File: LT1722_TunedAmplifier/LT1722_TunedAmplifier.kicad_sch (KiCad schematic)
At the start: 18 parts, among them U2 LT1722

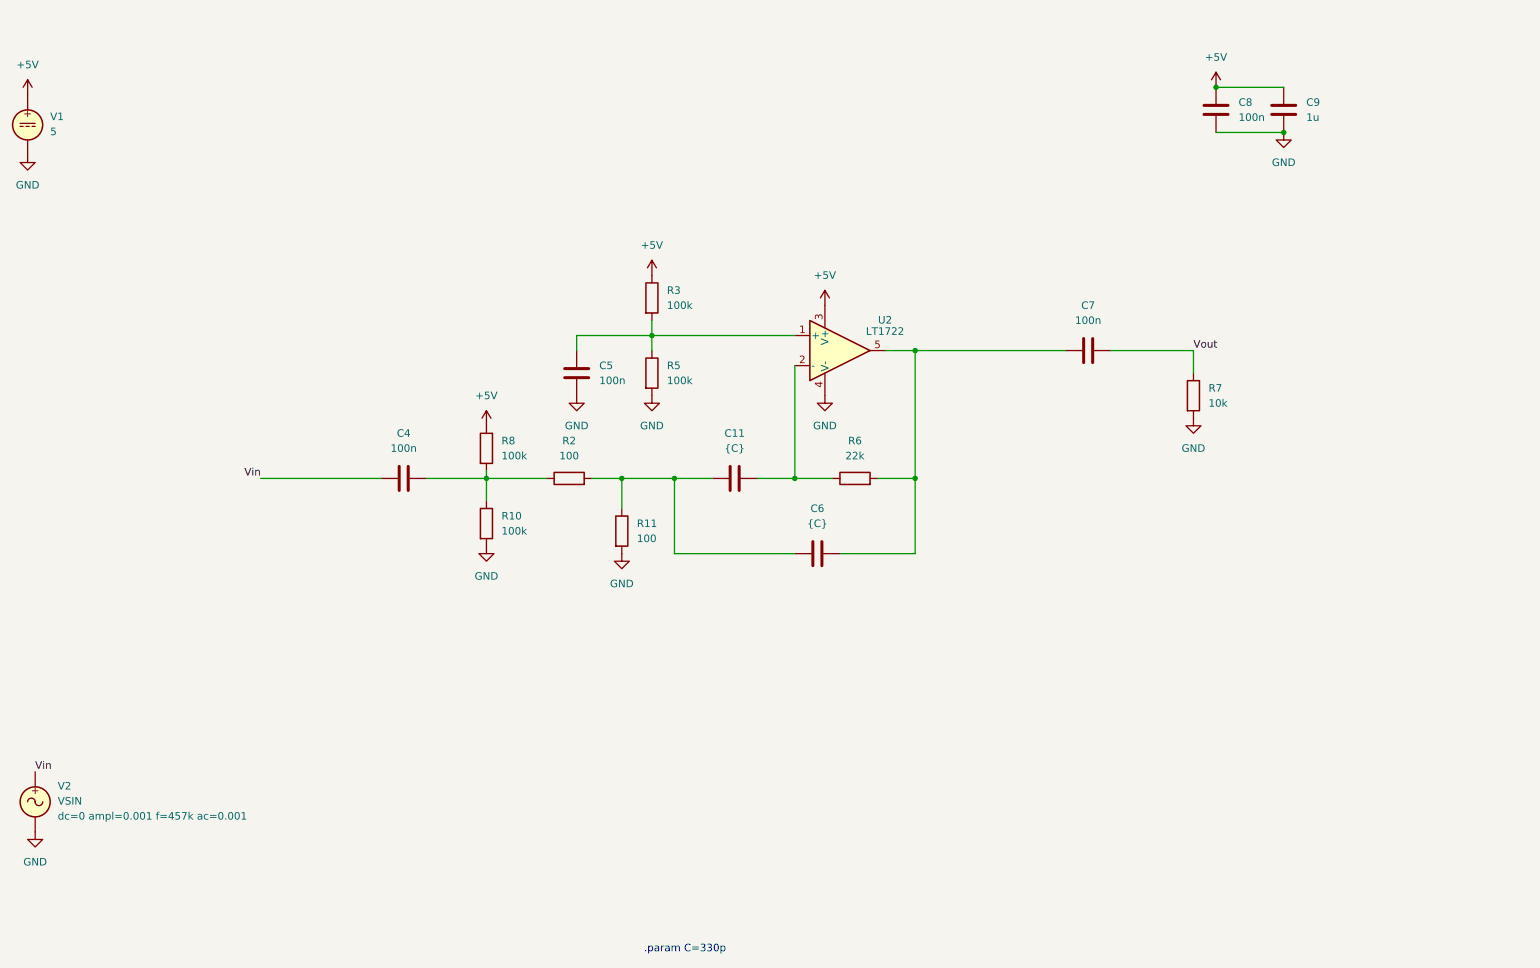
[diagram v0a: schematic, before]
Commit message: fix tuned amp
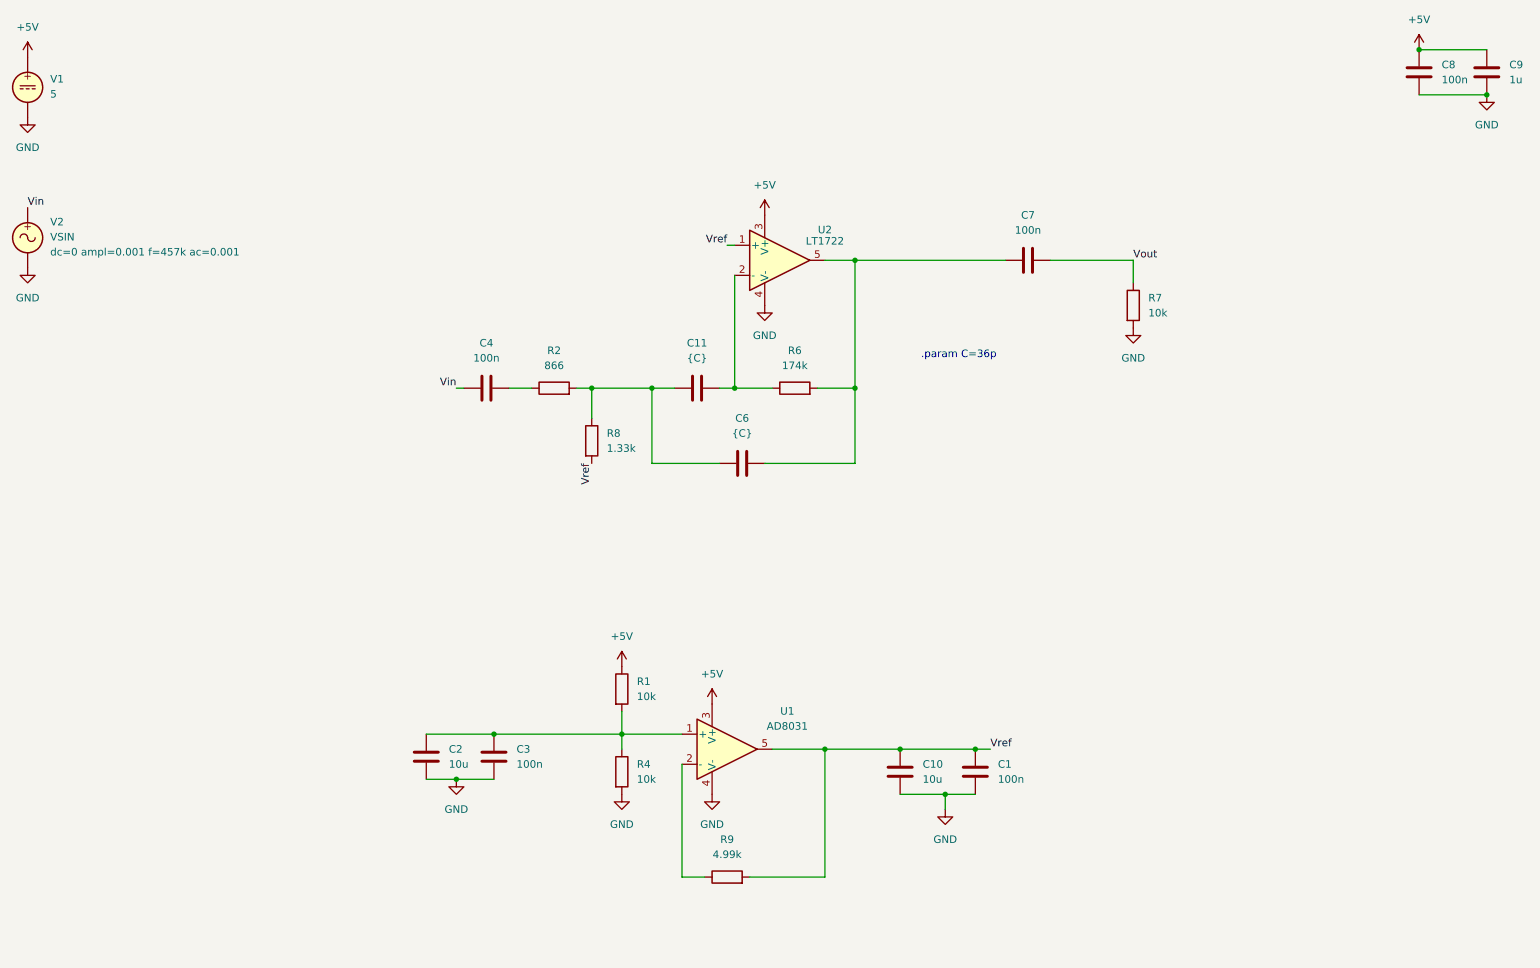
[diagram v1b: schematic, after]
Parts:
- removed C5: 100n, symbol Device:C
- removed R10, R3, R5: 100k, symbol Device:R
- removed R11: 100, symbol Device:R
- added C1, C3: 100n, symbol Device:C
- added C10, C2: 10u, symbol Device:C
- added R1, R4: 10k, symbol Device:R
- added R9: 4.99k, symbol Device:R
- added U1: AD8031, symbol Simulation_SPICE:OPAMP
- R2: value 100 -> 866
- R6: value 22k -> 174k
- R8: value 100k -> 1.33k
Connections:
- net +5V: now also R1.1, U1.3 (V+); no longer R8.1
- net GND: now also C1.2, C10.2, C2.2, C3.2, R4.2, U1.4 (V-)
- net at C4.2, R2.1: no longer R8.2
- net at C11.1, C6.1, R2.2: now also R8.1
- net Vref: now reaches U2.1 (+)
- net Vref: now also R8.2, C1.1, C10.1, R9.2, U1.5
- new net: C2.1, C3.1, R1.2, R4.1, U1.1 (+)
- new net: R9.1, U1.2 (-)
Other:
- note added: ".param C=36p"
- note removed: ".param C=330p"
- moved on the sheet: C11, C4, C6, C7, C8, C9, R2, R6, R7, U2, V1, V2
